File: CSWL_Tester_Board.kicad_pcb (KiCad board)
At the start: 2 copper layers, 210 parts, among them J1 Conn_02x10_Odd_Even, J2 Conn_01x03, J3 Conn_02x10_Odd_Even, J4 IDC 2.54mm, Q1 2N7002LT1G, Q2 2N7002LT1G, Q3 2N7002LT1G, Q4 2N7002LT1G, Q5 2N7002LT1G, Q6 2N7002LT1G, Q7 2N7002LT1G, Q8 2N7002LT1G, Q9 2N7002LT1G, U1 CD74HC4067M, U10 sn74hc595, U11 sn74hc595, U12 sn74hc595, U13 sn74hc595, U14 TCS3200, U15 TCS3200, U16 TCS3200, U17 TCS3200, U18 TCS3200, U19 TCS3200, U2 CD74HC4067M, U20 TCS3200, U21 TCS3200, U22 TCS3200, U23 TCS3200, U24 TCS3200, U25 TCS3200, U26 SN74HC151DR, U27 MCP1700T-3302E_TT, U28 SN74HC151DR, U29 74HC4016, U3 MCP1700T-3302E_TT, U4 sn74hc595, U5 sn74hc595, U6 sn74hc595, U7 STM32F103C8Tx, U8 sn74hc595, U9 sn74hc595, Y1 Crystal_GND24

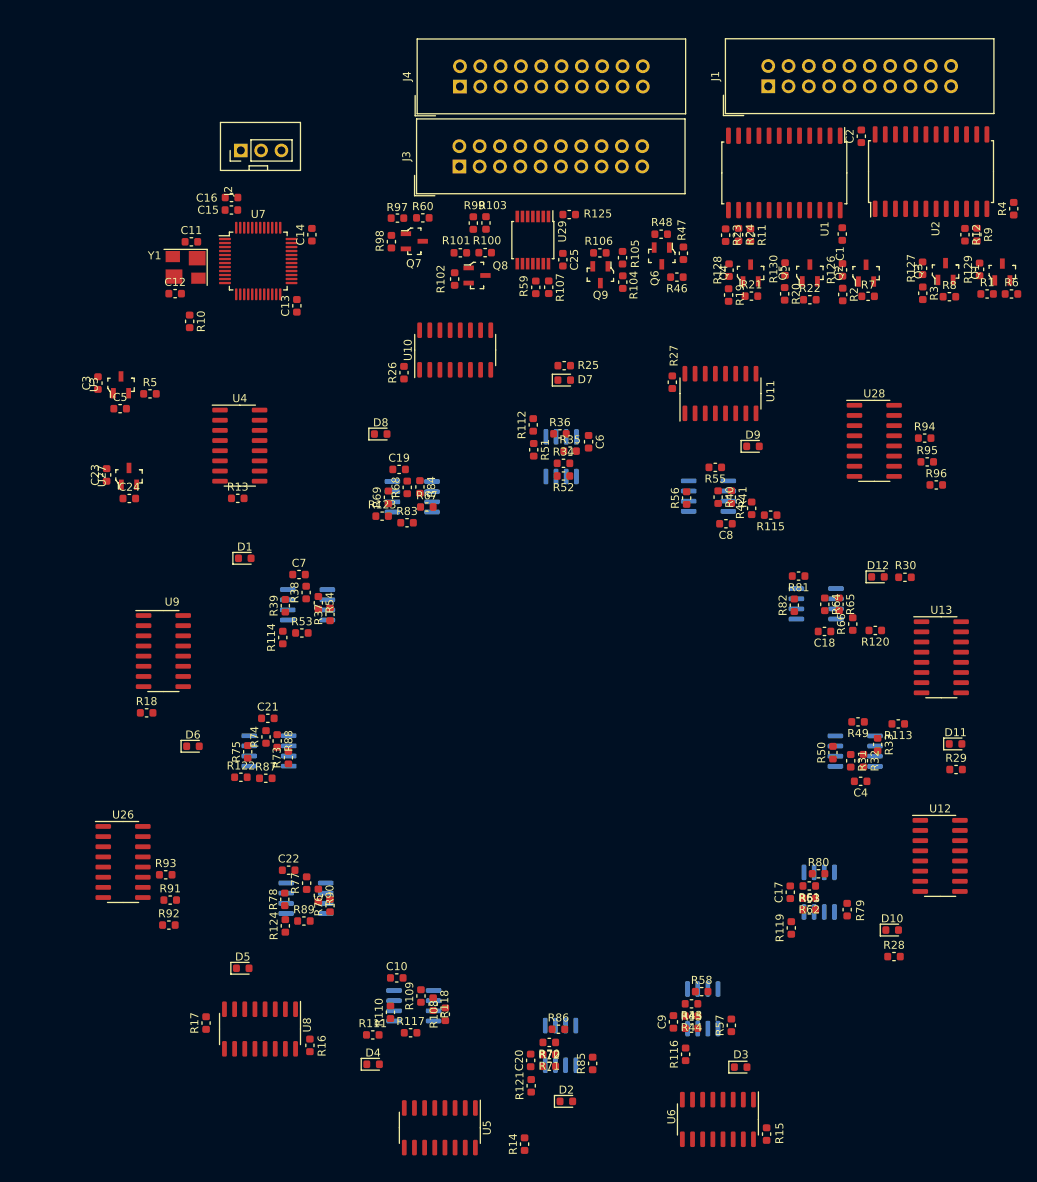
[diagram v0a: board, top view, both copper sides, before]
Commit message: Ruan: pcb designing
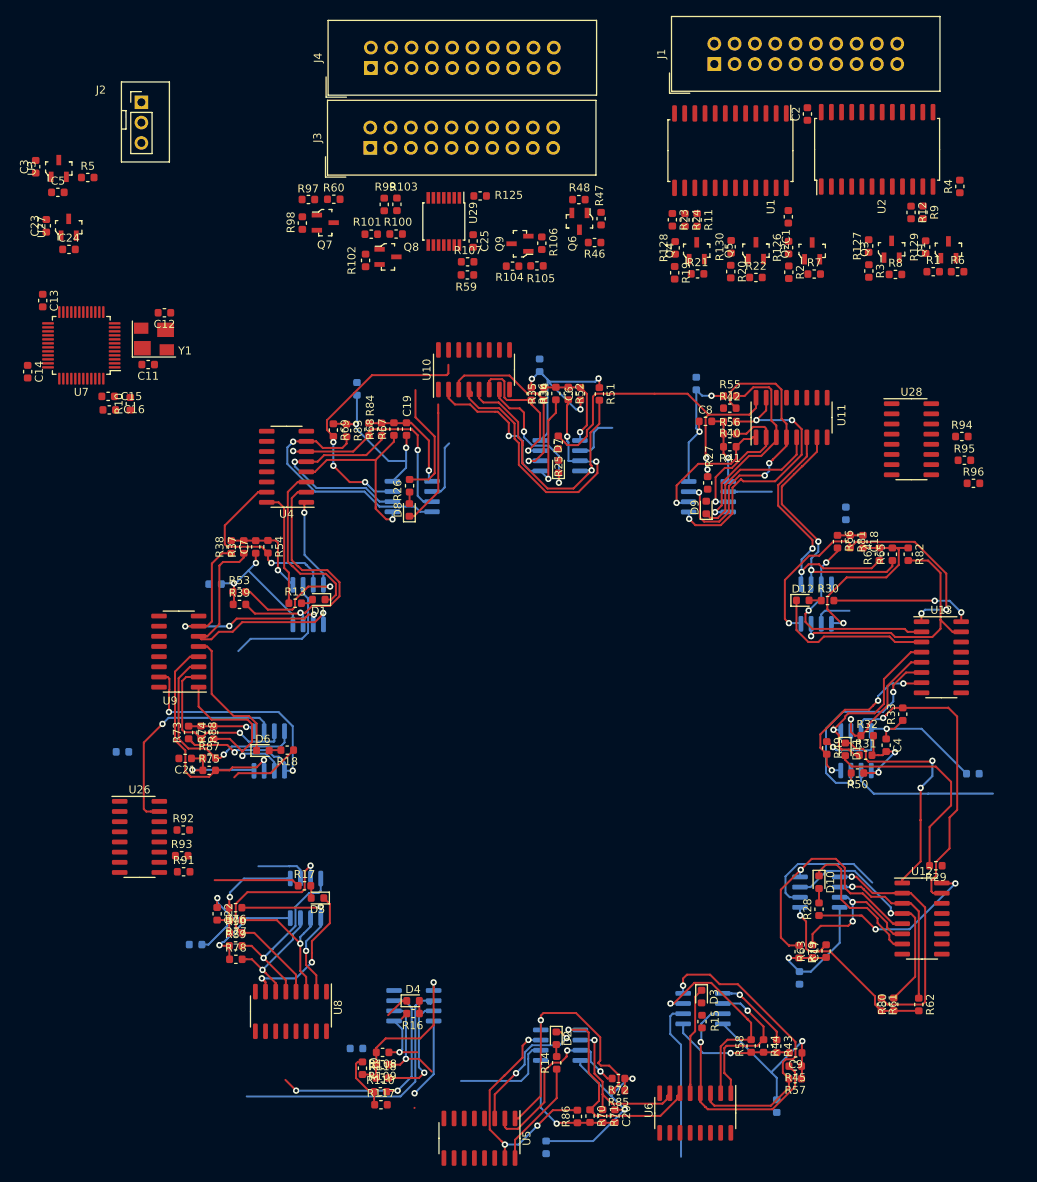
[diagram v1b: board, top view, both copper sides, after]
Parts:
- R111, R112, R113, R114, R115, R116, R119, R120, R121, R122, R123, R124: moved to B.Cu
- moved C14 39.4 mm to (90.5, 49.2), turned to 270 degrees
- moved C23 32.0 mm to (92.9, 31.0)
- moved C24 32.0 mm to (95.7, 33.9)
- moved U27 32.0 mm to (95.7, 31.1)
- moved C13 31.8 mm to (92.4, 40.3), turned to 270 degrees
- moved C16 30.6 mm to (100.7, 54.0), turned to 0 degrees
- moved U3 28.1 mm to (94.4, 23.8)
- moved C3 28.1 mm to (91.5, 23.6)
- moved C5 28.1 mm to (94.3, 26.8)
- moved R5 28.1 mm to (98.0, 24.9)
- moved C15 27.9 mm to (100.6, 52.3), turned to 0 degrees
- moved U7 24.5 mm to (97.2, 45.9), turned to 180 degrees
- moved R17 21.1 mm to (125.1, 113.5), turned to 0 degrees
- moved R62 19.1 mm to (201.9, 128.3), turned to 270 degrees
- moved R115 18.9 mm to (174.1, 50.7), turned to 270 degrees
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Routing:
- net GNDA: track 0.00 -> 226.8 mm, vias 0 -> 18
- net VCC33_B: track 0.00 -> 183.5 mm, vias 0 -> 13
- net VCC33_A: track 0.00 -> 144.4 mm, vias 0 -> 6
- net /LED5_S0: track 0.00 -> 42.9 mm, vias 0 -> 3
- net /LED10_S3: track 0.00 -> 40.8 mm, vias 0 -> 3
- net /LED8_S2: track 0.00 -> 39.7 mm, vias 0 -> 2
- net /LED1_S3: track 0.00 -> 39.1 mm, vias 0 -> 1
- net /LED11_EN: track 0.00 -> 38.9 mm, vias 0 -> 1
- net /LED9_EN: track 0.00 -> 38.7 mm, vias 0 -> 3
- net /LED9_S0: track 0.00 -> 36.3 mm, vias 0 -> 3
- net /LED8_S3: track 0.00 -> 34.9 mm, vias 0 -> 1
- net /LED3_OUT: track 0.00 -> 34.8 mm
- net /LED10_S1: track 0.00 -> 33.7 mm, vias 0 -> 2
- net /LED6_EN: track 0.00 -> 33.6 mm, vias 0 -> 1
- net /LED10_S2: track 0.00 -> 33.5 mm, vias 0 -> 1
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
